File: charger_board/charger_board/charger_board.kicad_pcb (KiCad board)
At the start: 2 copper layers, 110 x 20 mm, 37 parts, among them J1 Conn_01x04_Pin, J2 Conn_01x04_Pin, Q1 Si2319CDS, Q2 BC817, U1 STM32F042K6Tx, U2 PCA82C251, U3 LM317L_SOT-89

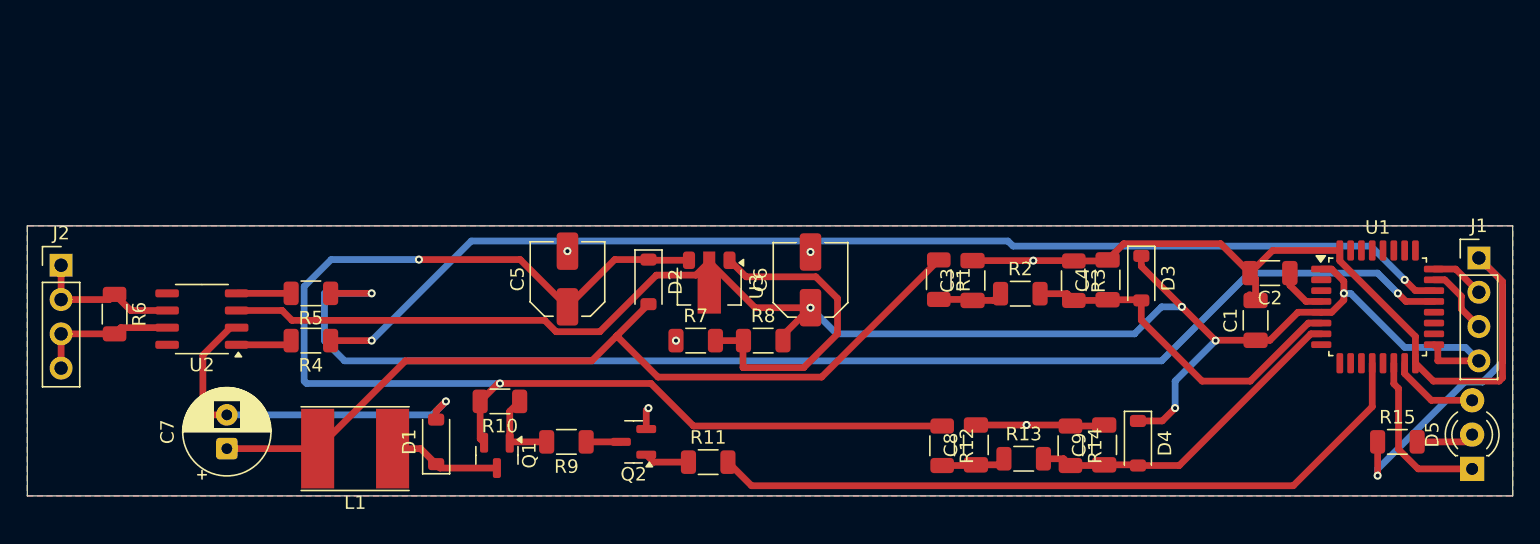
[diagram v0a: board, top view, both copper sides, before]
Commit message: placa bms pronta
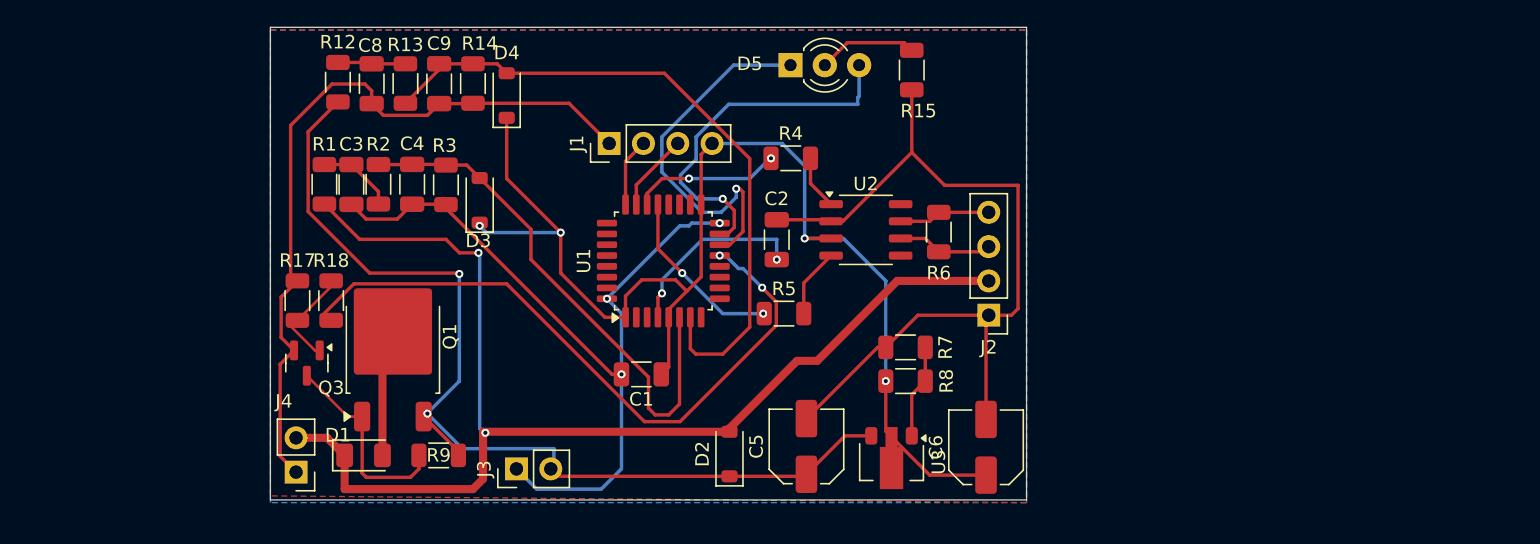
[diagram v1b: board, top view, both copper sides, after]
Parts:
- removed C7: 470uF, Capacitor_THT:CP_Radial_D6.3mm_P2.50mm
- removed L1: 680uH, Inductor_SMD:L_Taiyo-Yuden_NR-60xx_HandSoldering
- removed Q2: BC817, Package_TO_SOT_SMD:SOT-23
- removed R10: 10k, Resistor_SMD:R_1206_3216Metric
- removed R11: 1k, Resistor_SMD:R_1206_3216Metric
- added J3: Conn_01x02_Pin, Connector_PinHeader_2.54mm:PinHeader_1x02_P2.54mm_Vertical, F.Cu at (133.7, 112.5)
- added J4: Conn_01x02_Pin, Connector_PinHeader_2.54mm:PinHeader_1x02_P2.54mm_Vertical, F.Cu at (117.4, 112.7)
- added Q3: BC817, Package_TO_SOT_SMD:SOT-23, F.Cu at (118.2, 104.7)
- added R17: 10k, Resistor_SMD:R_1206_3216Metric, F.Cu at (117.5, 100.0)
- added R18: 1k, Resistor_SMD:R_1206_3216Metric, F.Cu at (120.0, 100.0)
- D1: value BAT42W-V -> 1N5405; footprint Diode_SMD:D_SOD-123 -> Diode_SMD:D_1206_3216Metric
- Q1: value Si2319CDS -> IRF9540N; footprint Package_TO_SOT_SMD:SOT-23 -> Package_TO_SOT_SMD:TO-252-2
- R14: value 3k3 -> 15K
- R3: value 1k2 -> 23K
- R9: value 4k7 -> 10k
- moved J2 68.8 mm to (168.7, 101.1), turned to 180 degrees
- moved J1 65.0 mm to (140.6, 88.4), turned to 90 degrees
- moved R6 61.3 mm to (165.0, 95.0), turned to 90 degrees
- moved D5 58.7 mm to (154.0, 82.6), turned to 0 degrees
- moved C9 56.0 mm to (128.0, 84.0), turned to -90 degrees
- moved R13 53.6 mm to (125.5, 84.0), turned to -90 degrees
- moved D4 53.4 mm to (133.0, 84.8), turned to 90 degrees
- moved U1 53.0 mm to (144.6, 97.1), turned to 90 degrees
- moved R12 52.2 mm to (120.5, 83.9), turned to 90 degrees
- moved C8 52.1 mm to (123.0, 84.0), turned to -90 degrees
- moved C4 52.0 mm to (126.0, 91.4), turned to -90 degrees
- moved R14 51.7 mm to (130.5, 84.0), turned to 90 degrees
- moved U2 49.6 mm to (159.6, 94.8), turned to 0 degrees
- moved D3 49.3 mm to (131.0, 92.6), turned to 90 degrees
- moved R2 48.2 mm to (123.5, 91.4), turned to 90 degrees
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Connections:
- C5 pad 1: +12V -> +5V
- D1 pad 1: Net-(D1-K) -> Lion_Batt
- D1 pad 2: GND -> Net-(D1-A)
- D2 pad 1: +12V -> +5V
- J2 pad 1: canl -> GND
- J2 pad 2: canl -> Lion_Batt
- J2 pad 3: canh -> canl
- Q1 pad 2: +12V -> Net-(D1-A)
- Q1 pad 3: Net-(D1-K) -> +5V
- R12 pad 1: +12V -> +5V
- R9 pad 1: Net-(Q2-C) -> Net-(Q1-G)
- R9 pad 2: Net-(Q1-G) -> +5V
- U1 pad 12: pwm_out_pa6 -> unconnected-(U1-PA6-Pad12)
- U1 pad 13: out_enable_pa7 -> charge_enable_pa7
- U1 pad 19: unconnected-(U1-PA9-Pad19) -> scl_sens_pa09
- U1 pad 20: unconnected-(U1-PA10-Pad20) -> sda_sens_pa10
- U3 pad 3: +12V -> +5V
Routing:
- net +12V: track 93.1 -> 0.00 mm, vias 2 -> 0
- net can_rx_pa11: track 96.4 -> 13.1 mm
- net can_tx_pa12: track 86.3 -> 11.0 mm
- net +5V: track 0.00 -> 75.1 mm, vias 0 -> 2
- net pwm_out_pa6: track 54.1 -> 0.00 mm
- net GND: track 122.5 -> 176.6 mm, vias 8 -> 3
- net charge_enable_pa7: track 0.00 -> 49.0 mm, vias 0 -> 2
- net +3V3: track 127.7 -> 93.2 mm, vias 5 -> 4
- net Lion_Batt: track 64.4 -> 89.6 mm, vias 0 -> 2
- net charger_in_pa1: track 24.9 -> 50.1 mm
- net led_green_pa2: track 7.09 -> 27.1 mm, vias 0 -> 1
- net Net-(U3-ADJ): track 23.9 -> 6.96 mm
- net led_red_pa3: track 13.1 -> 27.8 mm, vias 0 -> 1
- net batt_med_pa0: track 26.2 -> 39.4 mm
- net Net-(U1-NRST): track 3.72 -> 14.1 mm, vias 0 -> 2
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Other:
- board size 110 x 20 mm -> 56 x 35 mm
